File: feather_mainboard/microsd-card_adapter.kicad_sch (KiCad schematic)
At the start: 10 parts, among them J2 MEM2090-00-145-00-A

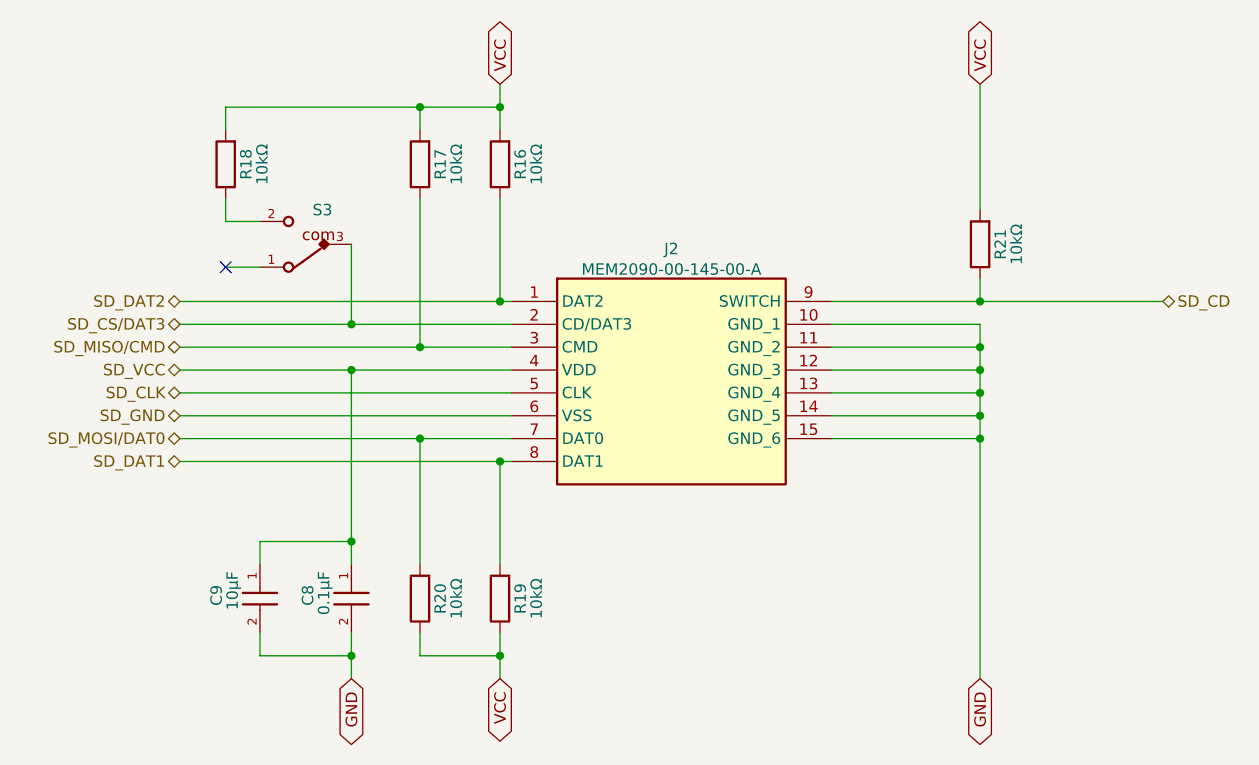
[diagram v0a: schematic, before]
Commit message: schematic is almost done (check TODOs in schematic file)
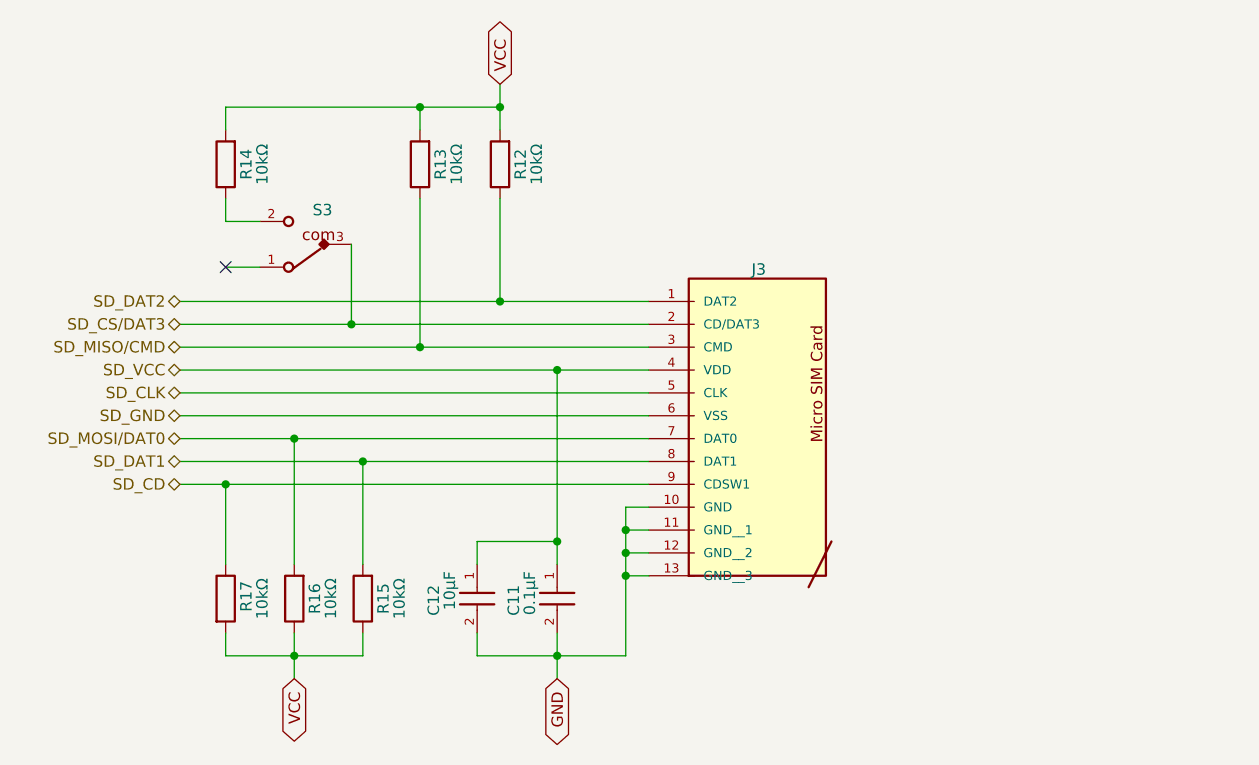
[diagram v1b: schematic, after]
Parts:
- removed J2: MEM2090-00-145-00-A, Custom footprints:MEM20900014500A, symbol MEM2090-00-145-00-A:MEM2090-00-145-00-A
- removed R19, R20, R21: 10kΩ, Resistor_SMD:R_0805_2012Metric_Pad1.20x1.40mm_HandSolder, symbol Device:R
- added J3: 693071020811, Custom footprints:693071020811, symbol 693071020811:693071020811
- added R15, R16, R17: 10kΩ, Resistor_SMD:R_0805_2012Metric_Pad1.20x1.40mm_HandSolder, symbol Device:R
- renumbered C8 to C11, C9 to C12, R16 to R12, R17 to R13, R18 to R14
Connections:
- net GND: now also J3.10 (GND), J3.11 (GND__1), J3.12 (GND__2), J3.13 (GND__3)
- net SD_CD: now also J3.9 (CDSW1), R17.1
- net SD_CLK: now also J3.5 (CLK)
- net SD_CS/DAT3: now also J3.2 (CD/DAT3)
- net SD_DAT1: now also J3.8 (DAT1), R15.2
- net SD_DAT2: now also J3.1 (DAT2)
- net SD_GND: now also J3.6 (VSS)
- net SD_MISO/CMD: now also J3.3 (CMD)
- net SD_MOSI/DAT0: now also J3.7 (DAT0), R16.2
- net SD_VCC: now also J3.4 (VDD)
- net VCC: now also R15.1, R16.1, R17.2
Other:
- moved on the sheet: C11, C12
